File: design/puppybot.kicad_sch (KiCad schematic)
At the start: 11 parts, among them M1 Motor_DC, M2 Motor_DC, M5 Motor_DC, M6 Motor_DC, U1 L298N, U2 ESP32-C3-WROOM-02, U3 LM2596S-12, U4 L298N

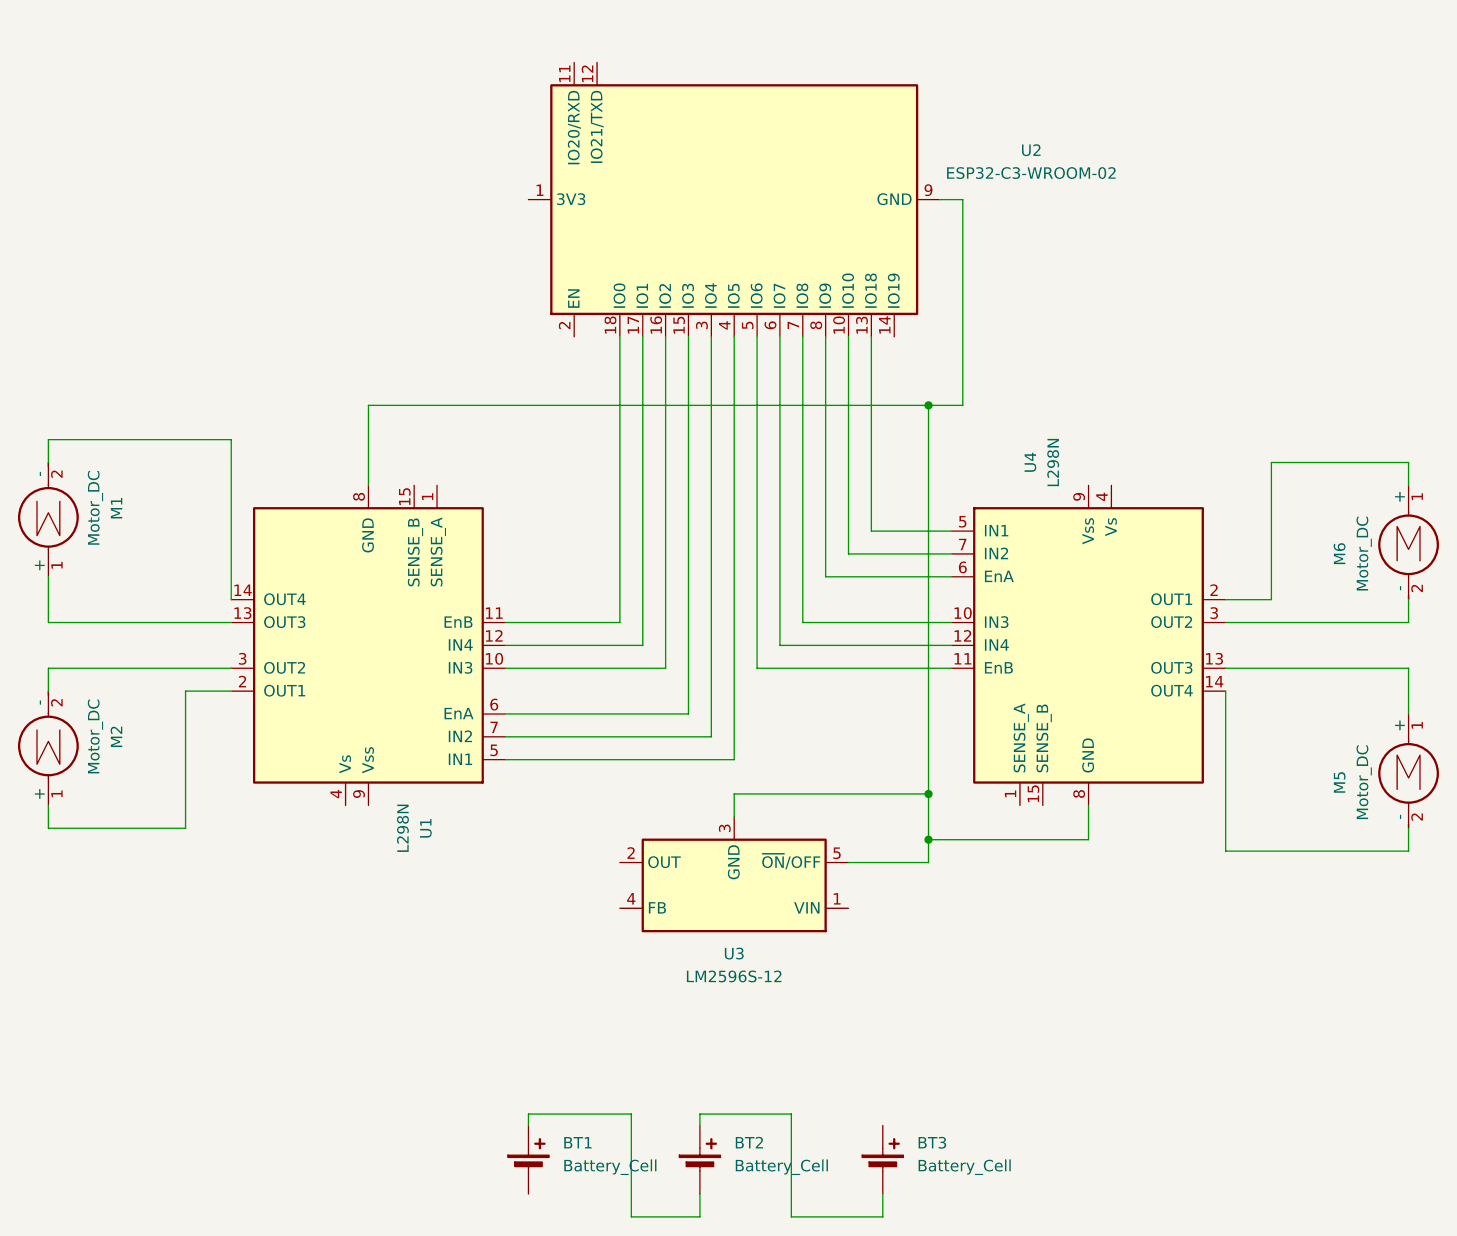
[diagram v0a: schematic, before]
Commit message: update elecric design
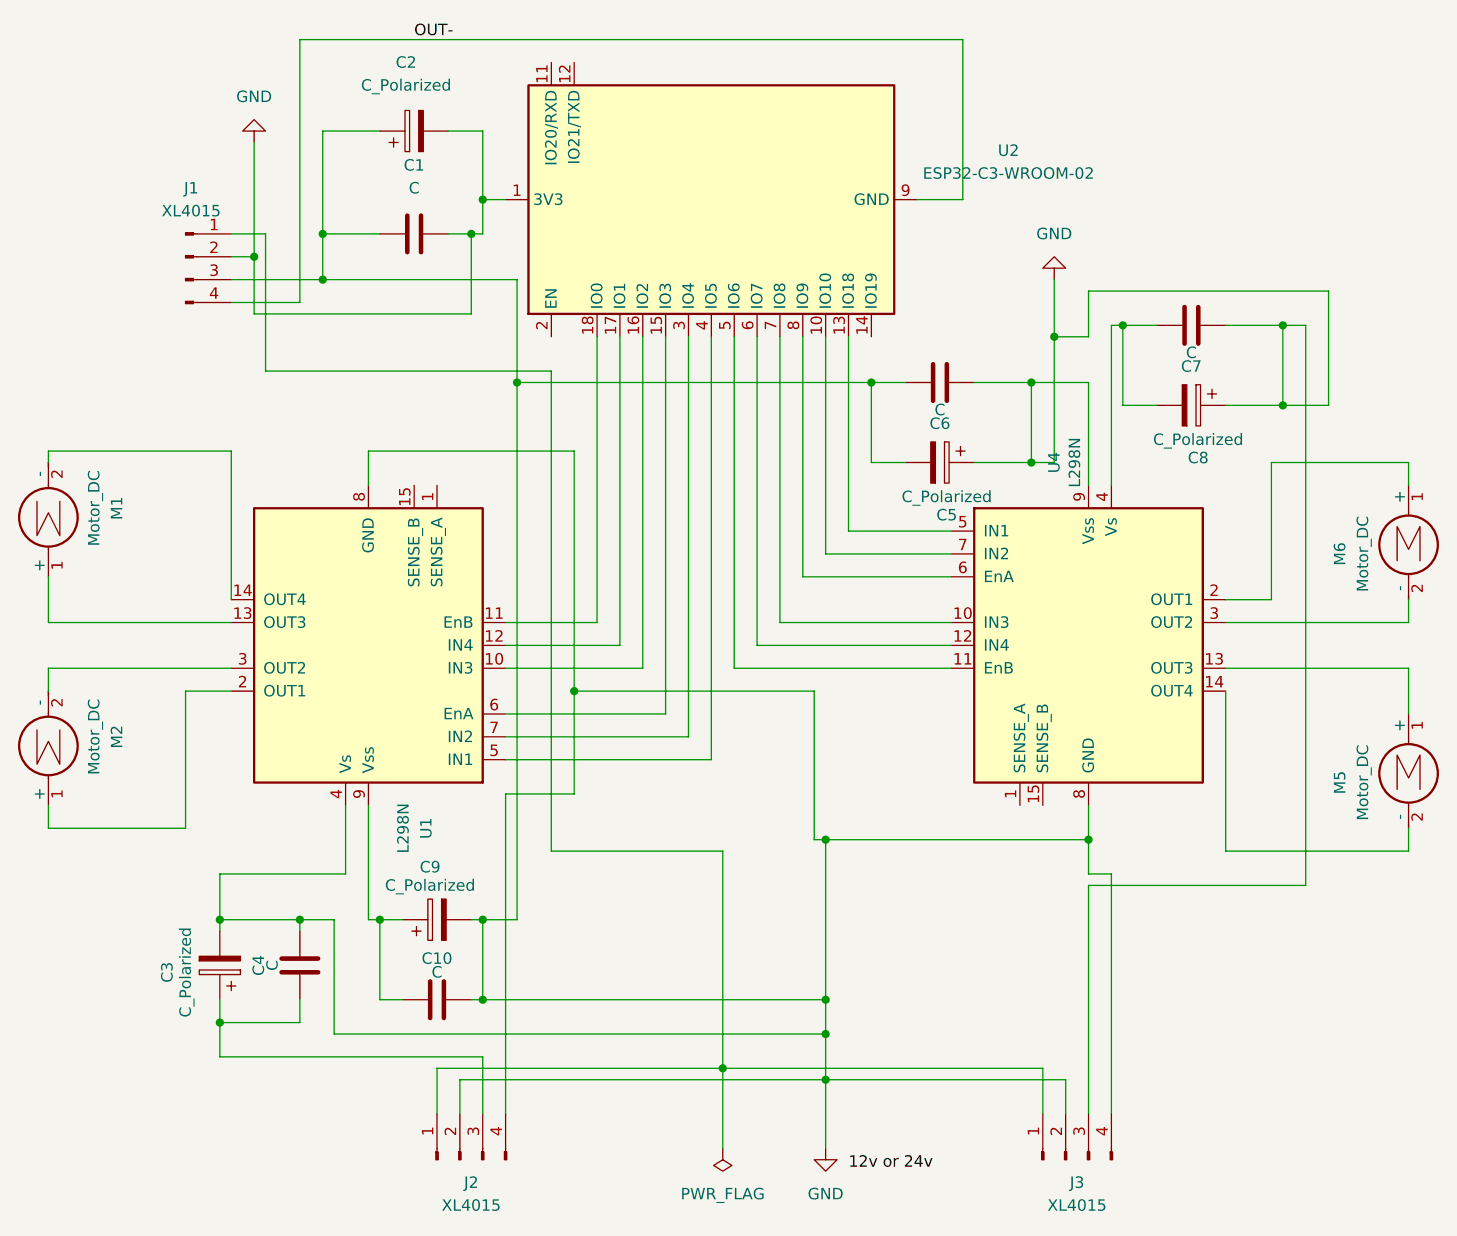
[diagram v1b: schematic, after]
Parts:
- removed BT1, BT2, BT3: Battery_Cell, symbol Device:Battery_Cell
- removed U3: LM2596S-12, Package_TO_SOT_SMD:TO-263-5_TabPin3, symbol Regulator_Switching:LM2596S-12
- added C1, C10, C4, C6, C7: C, Capacitor_SMD:C_0805_2012Metric, symbol Device:C
- added C2, C3, C5, C8, C9: C_Polarized, Capacitor_THT:CP_Radial_D5.0mm_P2.00mm, symbol Device:C_Polarized
- added J1, J2, J3: XL4015, Connector:FanPinHeader_1x04_P2.54mm_Vertical, symbol Connector:Conn_01x04_Pin
- M1, M2, M5, M6: footprint (none) -> TerminalBlock_RND:TerminalBlock_RND_205-00234_1x04_P5.08mm_Horizontal
- U1, U4: footprint Package_TO_SOT_THT:TO-220-15_P2.54x2.54mm_StaggerOdd_Lead4.58mm_Vertical -> Package_DIP:DIP-16_W7.62mm
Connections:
- net GND: now reaches U2.1 (3V3)
- net GND: now also U1.4 (Vs), U1.8 (GND), U4.8 (GND), U4.9 (Vss), C1.1, C1.2, C10.2, C2.1, C2.2, C3.2, C4.2, C5.1, C5.2, C6.1, C6.2, C7.1, C8.1, C9.2, J1.2 (Pin_2), J1.3 (Pin_3), J2.2 (Pin_2), J2.4 (Pin_4), J3.2 (Pin_2), J3.3 (Pin_3), J3.4 (Pin_4)
- net OUT-: now reaches U2.19 (GND), U2.9 (GND)
- net OUT-: now also J1.4 (Pin_4); no longer U1.8 (GND), U4.8 (GND)
- net at U4.4 (Vs): now also C7.2, C8.2
- net at U1.9 (Vss): now also C10.1, C9.1
- new net: J1.1 (Pin_1), J2.1 (Pin_1), J3.1 (Pin_1)
- new net: C3.1, C4.1, J2.3 (Pin_3)
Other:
- moved on the sheet: U2
